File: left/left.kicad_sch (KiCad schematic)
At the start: 19 parts, among them J1 USB_C_Receptacle_IN, J2 USB_C_Receptacle_OUT, SW1 SW_Push, SW2 SW_SPDT, U1 STM32G0B1CBTx, U2 SRV05-4, U3 XC6206P332MR, U4 SRV05-4

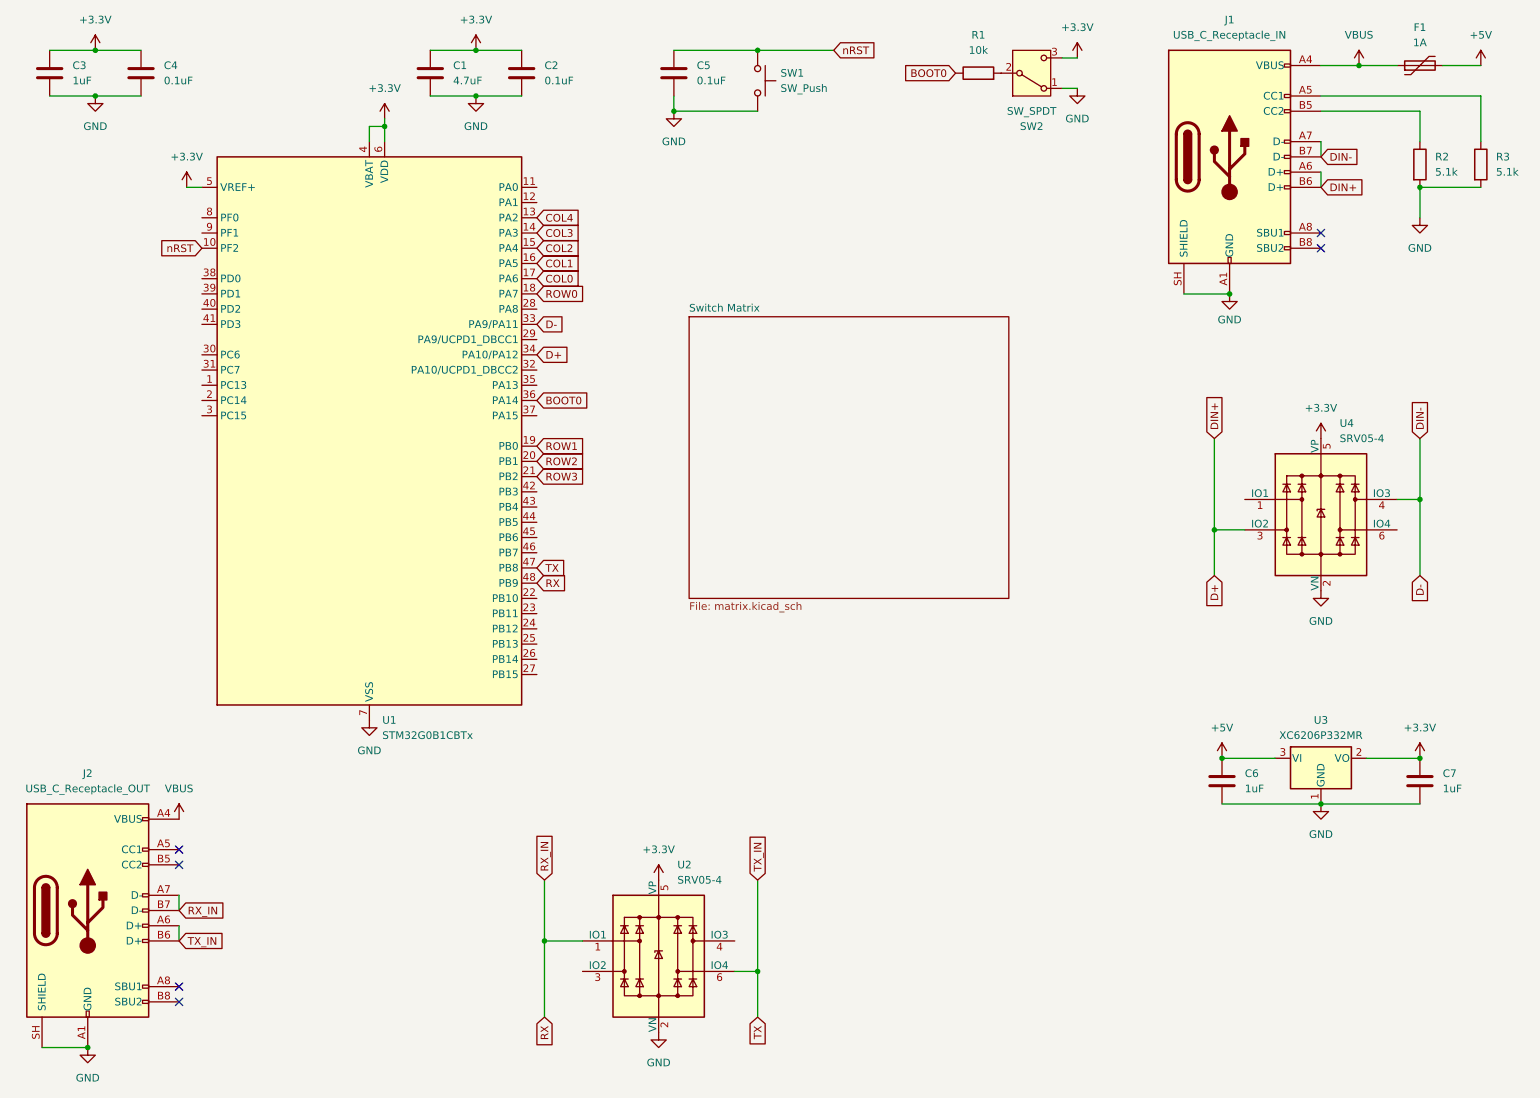
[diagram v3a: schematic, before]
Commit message: v3 for left
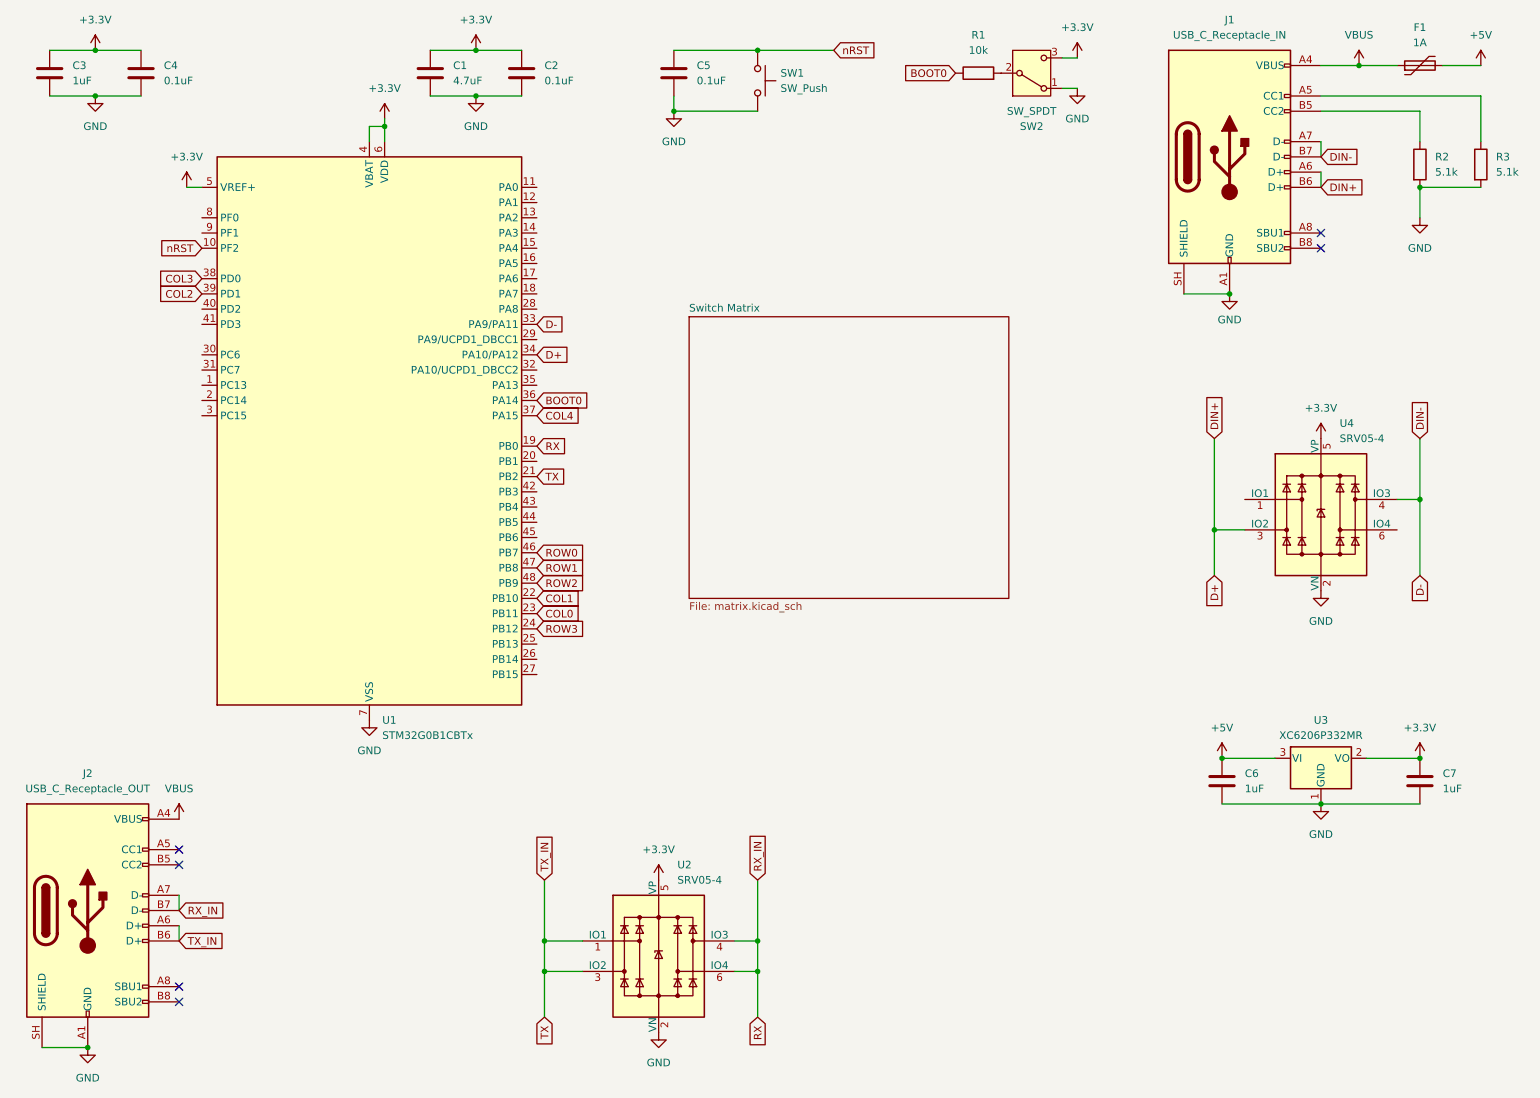
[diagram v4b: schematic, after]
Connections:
- net COL0: now also U1.23 (PB11); no longer U1.17 (PA6)
- net COL1: now also U1.22 (PB10); no longer U1.16 (PA5)
- net COL2: now also U1.39 (PD1); no longer U1.15 (PA4)
- net COL3: now also U1.38 (PD0); no longer U1.14 (PA3)
- net COL4: now also U1.37 (PA15); no longer U1.13 (PA2)
- net ROW0: now also U1.46 (PB7); no longer U1.18 (PA7)
- net ROW1: now also U1.47 (PB8); no longer U1.19 (PB0)
- net ROW2: now also U1.48 (PB9); no longer U1.20 (PB1)
- net ROW3: now also U1.24 (PB12); no longer U1.21 (PB2)
- net RX: now also U1.19 (PB0), U2.4 (IO3), U2.6 (IO4); no longer U1.48 (PB9), U2.1 (IO1)
- net TX: now also U1.21 (PB2), U2.1 (IO1), U2.3 (IO2); no longer U1.47 (PB8), U2.6 (IO4)
